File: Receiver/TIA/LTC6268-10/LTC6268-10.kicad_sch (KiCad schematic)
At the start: 28 parts, among them J1 IN, J2 Vout, J3 TEST, J4 OUT, U1 LTC6268-10-SOT23

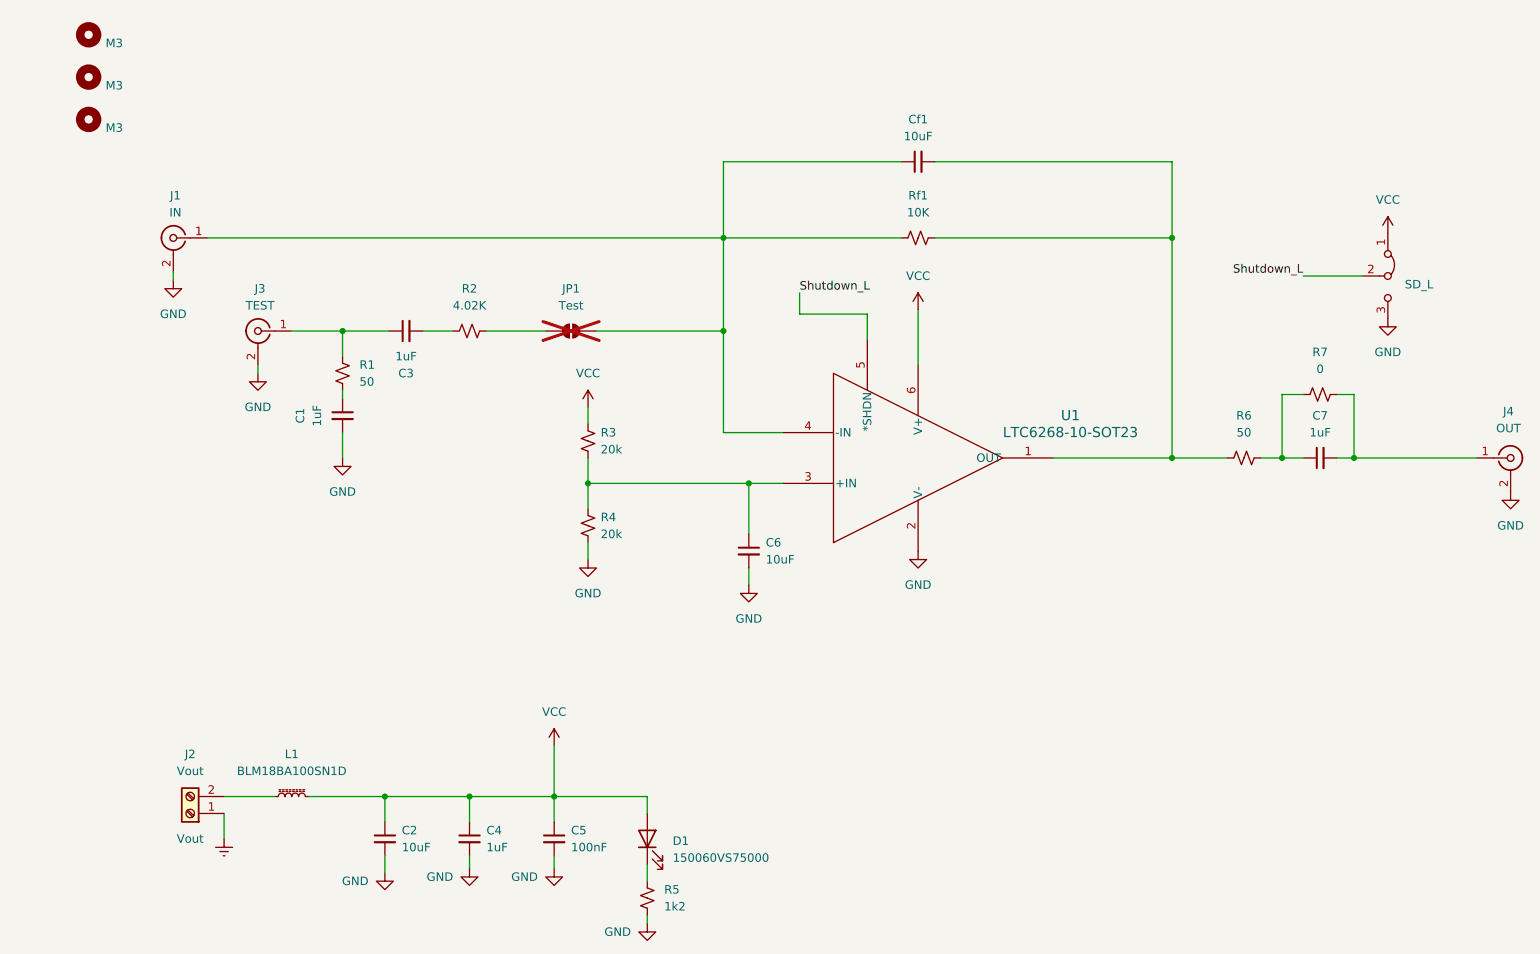
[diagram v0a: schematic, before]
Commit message: LTC6268-10 first version
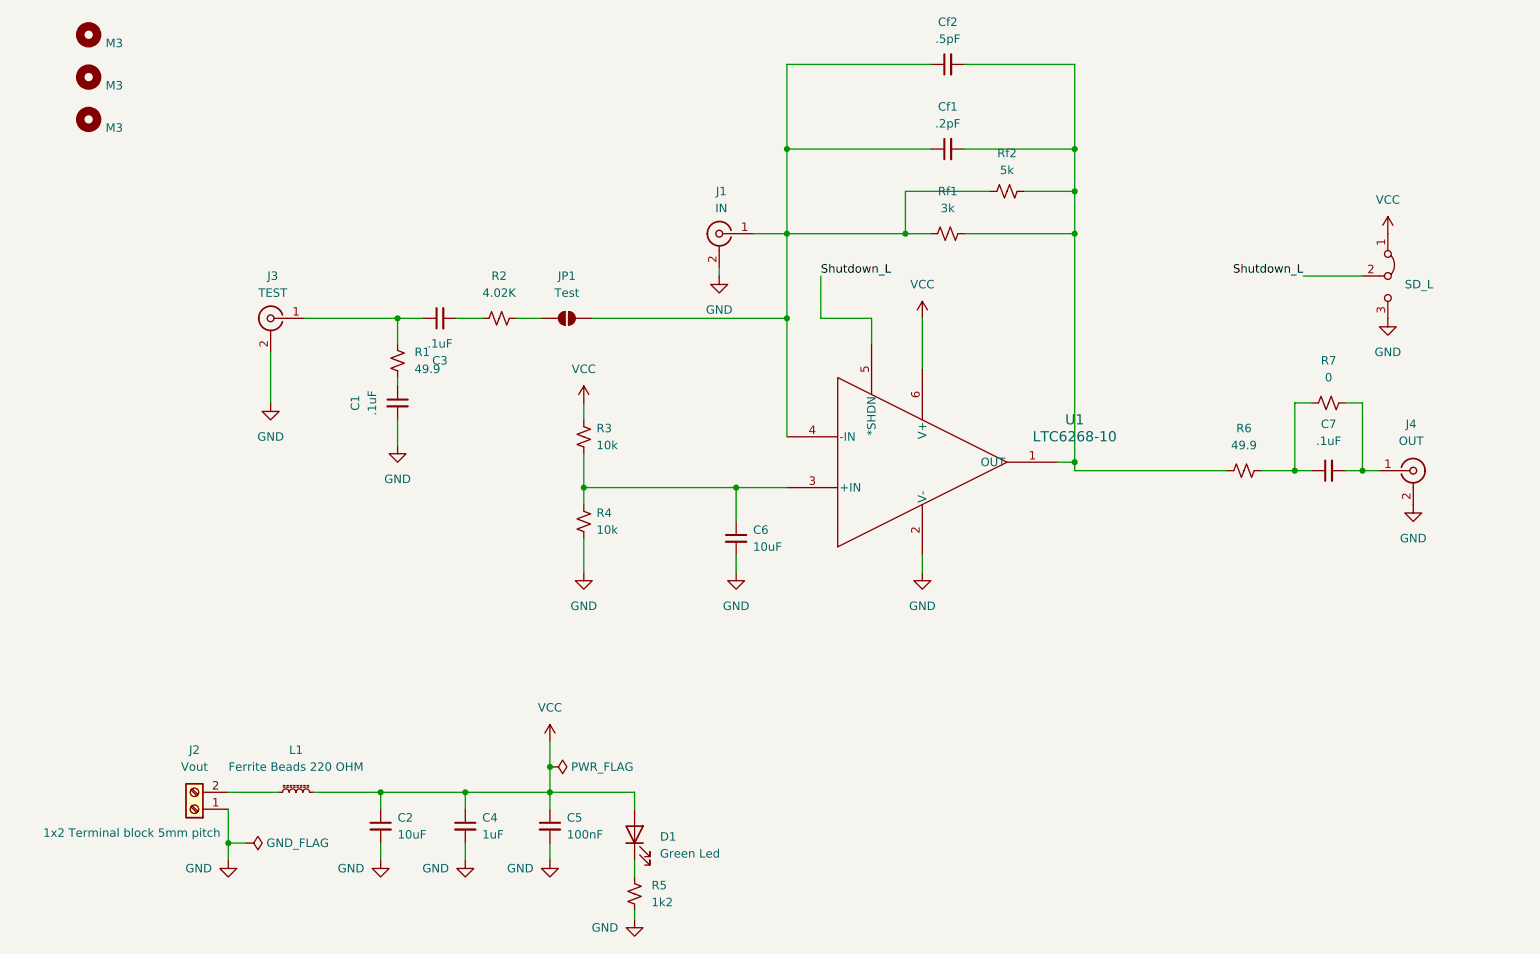
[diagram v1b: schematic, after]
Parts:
- added Cf2: .5pF, Capacitor_SMD:C_0402_1005Metric, symbol Device:C_Small
- added Rf2: 5k, Resistor_SMD:R_0402_1005Metric, symbol Device:R_Small_US
- C1, C3, C7: value 1uF -> .1uF; footprint Capacitor_SMD:C_0603_1608Metric_Pad1.08x0.95mm_HandSolder -> Capacitor_SMD:C_0402_1005Metric_Pad0.74x0.62mm_HandSolder; Manufacturer (none) -> KYOCERA AVX; Manufacturer Part Number (none) -> 530L104KT16; Mouser Part Number (none) -> 581-530L104KT16
- C2, C6: Manufacturer (none) -> Murata Electronics; Manufacturer Part Number (none) -> GRM188Z71A106MA73D; Mouser Part Number (none) -> 81-GRM188Z71A106MA3D
- C4: Manufacturer (none) -> Samsung Electro-Mechanics; Manufacturer Part Number (none) -> CL10B105KP8NNNC; Mouser Part Number (none) -> 187-CL10B105KP8NNNC
- C5: Manufacturer (none) -> Samsung Electro-Mechanics; Manufacturer Part Number (none) -> CL10B104KO8NFNC; Mouser Part Number (none) -> 187-CL10B104KO8NFNC
- Cf1: value 10uF -> .2pF; footprint Capacitor_SMD:C_0603_1608Metric_Pad1.08x0.95mm_HandSolder -> Capacitor_SMD:C_0402_1005Metric; Manufacturer (none) -> KYOCERA AVX; Manufacturer Part Number (none) -> 04023J0R2ZBSTR; Mouser Part Number (none) -> 581-04023J0R2ZBSTR
- D1: value 150060VS75000 -> Green Led; footprint LumiCom_TIA:LEDC1608X80N -> LED_SMD:LED_0603_1608Metric; Manufacturer (none) -> Wurth Elektronik; Manufacturer Part Number (none) -> 150060VS75000; Mouser Part Number (none) -> 710-150060VS75000
- JP1: now fitted; now in the parts list
- L1: value BLM18BA100SN1D -> Ferrite Beads 220 OHM; Manufacturer (none) -> Murata Electronics; Manufacturer Part Number (none) -> BLM18KG221SN1D; Mouser Part Number (none) -> 81-BLM18KG221SN1D
- R1, R6: value 50 -> 49.9; Manufacturer (none) -> Vishay / Beyschlag; Manufacturer Part Number (none) -> MCT06030C4999FP500; Mouser Part Number (none) -> 594-MCT06030C4999FP5
- R2: Manufacturer (none) -> Vishay / Beyschlag; Manufacturer Part Number (none) -> MCT06030C4021FP500; Mouser Part Number (none) -> 594-MCT06030C4021FP5
- R3, R4: value 20k -> 10k; Manufacturer (none) -> Vishay / Dale; Manufacturer Part Number (none) -> CRCW060310K0FKEI; Mouser Part Number (none) -> 71-CRCW060310K0FKEI
- R5: Manufacturer (none) -> Vishay / Dale; Manufacturer Part Number (none) -> CRCW08051K20FKEAC; Mouser Part Number (none) -> 71-CRCW08051K20FKEAC
- R7: Manufacturer (none) -> Vishay / Beyschlag; Manufacturer Part Number (none) -> MCT0603MZ0000ZP500; Mouser Part Number (none) -> 594-MCT0603MZ0000ZP5
- Rf1: value 10K -> 3k; footprint Resistor_SMD:R_0603_1608Metric_Pad0.98x0.95mm_HandSolder -> Resistor_SMD:R_0402_1005Metric; Manufacturer (none) -> Vishay; Manufacturer Part Number (none) -> MCS04020D3001BE000; Mouser Part Number (none) -> 594-MCS04020D3001BE0
- U1: value LTC6268-10-SOT23 -> LTC6268-10; Manufacturer (none) -> Analog Devices; Manufacturer Part Number (none) -> LTC6268IS6-10#TRMPBF; Mouser Part Number (none) -> 584-C6268IS6-10TMPF
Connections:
- net at Cf1.1, J1.1 (In), JP1.2 (B)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: now also Cf2.1, Rf2.1
- net at Cf1.2, R6.1, Rf1.2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: now also Cf2.2, Rf2.2
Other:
- moved on the sheet: C1, C2, C3, C4, C5, C6, C7, Cf1, D1, J1, J2, J3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

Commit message: LMH3440 fixed
LMH3440 fixed
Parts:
- R5: Manufacturer Vishay / Dale -> Vishay / Dale; Manufacturer Part Number CRCW08051K20FKEAC -> CRCW06031K20FKEA; Mouser Part Number 71-CRCW08051K20FKEAC -> 71-CRCW0603-1.2K-E3
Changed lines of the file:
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@@
 			)
 		)
-		(property "Datasheet" "https://www.vishay.com/doc?28773"
+		(property "Datasheet" "https://www.vishay.com/doc?20035"
 			(at 124.46 175.26 0)
 			(effects
@@
 			)
 		)
-		(property "Description" "1/8Watt 1.2Kohms 1% Commercial Use"
+		(property "Description" " Thick Film Resistors - SMD 1/10watt 1.2Kohms 1% 0603"
 			(at 124.46 175.26 0)
 			(effects
@@
 			)
 		)
-		(property "Manufacturer" "Vishay / Dale"
+		(property "Manufacturer" " Vishay / Dale "
 			(at 124.46 175.26 0)
 			(effects
@@
 			)
 		)
-		(property "Manufacturer Part Number" "CRCW08051K20FKEAC"
+		(property "Manufacturer Part Number" " CRCW06031K20FKEA "
 			(at 124.46 175.26 0)
 			(effects
@@
 			)
 		)
-		(property "Mouser Part Number" " 71-CRCW08051K20FKEAC "
+		(property "Mouser Part Number" " 71-CRCW0603-1.2K-E3 "
 			(at 124.46 175.26 0)
 			(effects

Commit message: Fixed missing symbol LTC6268-10
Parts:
- JP1: Manufacturer (none) -> Vishay / Beyschlag; Manufacturer Part Number (none) -> MCT0603MZ0000ZP500; Mouser Part Number (none) -> 594-MCT0603MZ0000ZP5
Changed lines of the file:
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@@
 			)
 		)
-		(property "Datasheet" "~"
+		(property "Datasheet" "https://www.vishay.com/doc?28952"
 			(at 114.3 88.9 0)
 			(effects
@@
 			)
 		)
-		(property "Description" "Solder Jumper, 2-pole, open"
+		(property "Description" " Thin Film Resistors .1W ZEROohm Jumper "
 			(at 114.3 88.9 0)
 			(effects
@@
 			)
 		)
-		(property "Manufacturer" ""
+		(property "Manufacturer" " Vishay / Beyschlag "
 			(at 114.3 88.9 0)
 			(effects
@@
 			)
 		)
-		(property "Manufacturer Part Number" ""
+		(property "Manufacturer Part Number" " MCT0603MZ0000ZP500 "
 			(at 114.3 88.9 0)
 			(effects
@@
 			)
 		)
-		(property "Mouser Part Number" ""
+		(property "Mouser Part Number" " 594-MCT0603MZ0000ZP5 "
 			(at 114.3 88.9 0)
 			(effects
